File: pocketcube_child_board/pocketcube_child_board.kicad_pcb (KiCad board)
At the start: 4 copper layers, 47 x 47 mm, 17 parts, among them J1 M55-7102642R, J2 M55-7101242R, J3 M55-7101242R, J4 M55-7101242R, U1 SI3477DV-T1-GE3

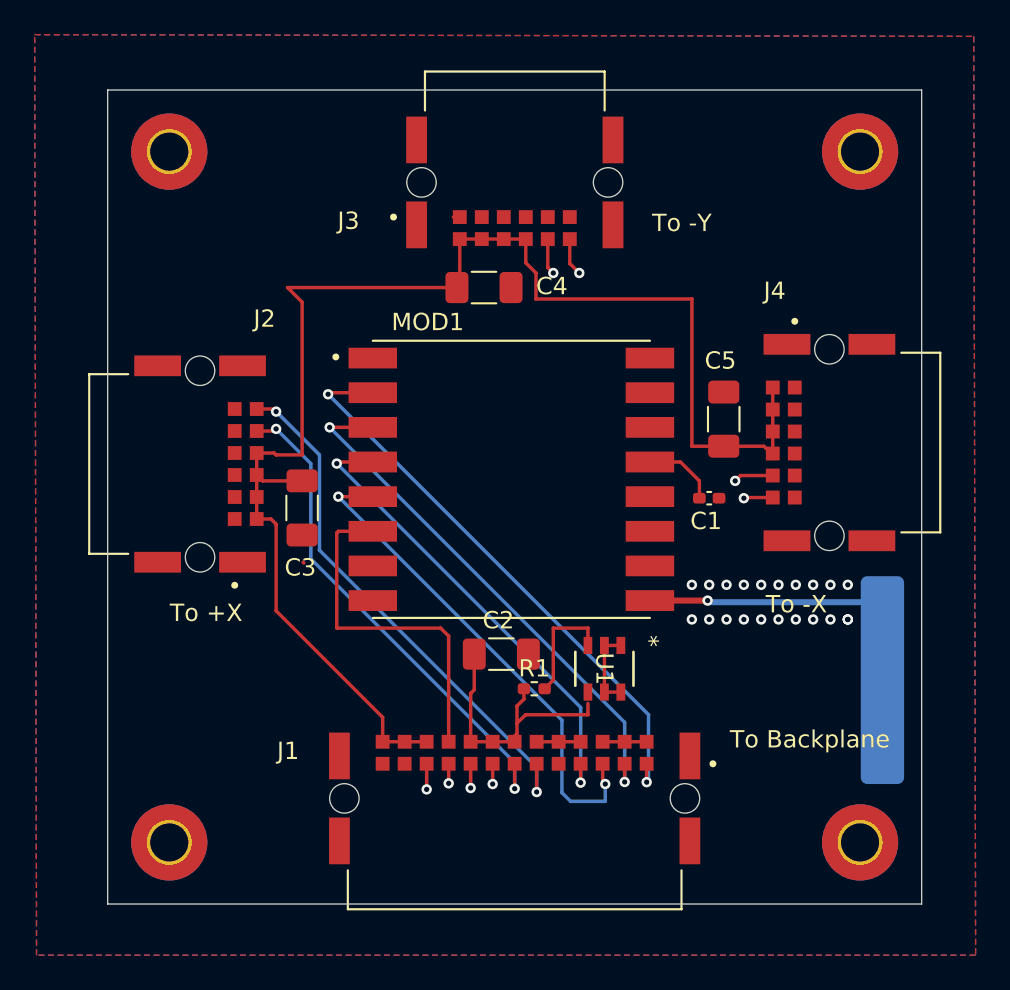
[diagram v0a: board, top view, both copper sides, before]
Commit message: Pushing Routing Changes
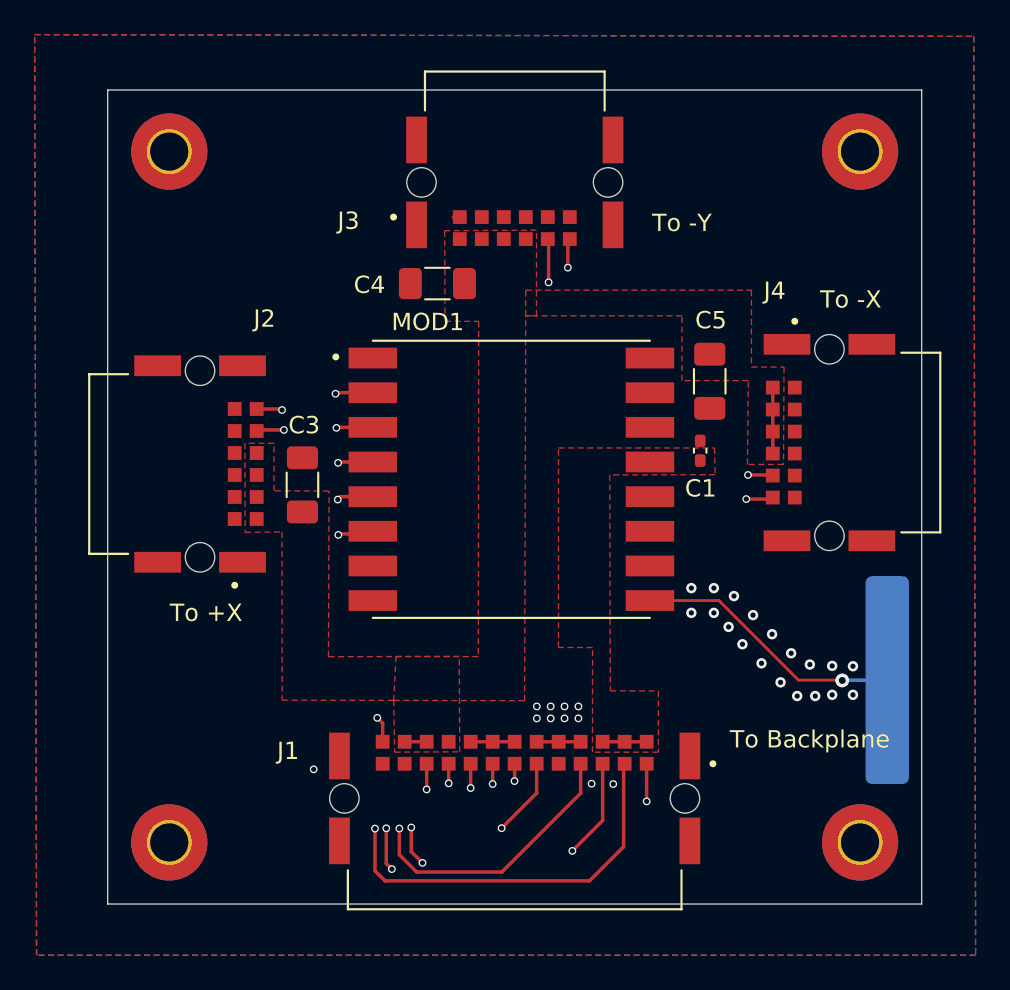
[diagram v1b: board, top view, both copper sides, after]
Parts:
- removed C2: 47uF, Capacitor_SMD:C_1206_3216Metric_Pad1.33x1.80mm_HandSolder
- removed R1: 100K, Resistor_SMD:R_0402_1005Metric_Pad0.72x0.64mm_HandSolder
- removed U1: SI3477DV-T1-GE3, inspirefly:SOT_V-T1-GE3_VIS
- moved C1 2.79 mm to (235.0, 54.8), turned to -90 degrees
- moved C4 2.70 mm to (219.8, 45.1), turned to 0 degrees
- moved C5 2.33 mm to (235.5, 50.8), turned to 90 degrees
- moved C3 1.33 mm to (212.0, 56.7), turned to -90 degrees
- moved AE1 0.28 mm to (252.5, 68.0)
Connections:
- C1 pad 2: 3.3V -> +3.3V
- J1 pad A1: ANT_SPI2_MISO -> ANT_SPI2_MOSI
- J1 pad A2: ANT_SPI2_MOSI -> ANT_SPI2_MISO
- J1 pad B10: RFM_RESET -> EXTERNAL_VOLTAGE
- J1 pad B13: EXTERNAL_VOLTAGE -> RFM_RESET
- MOD1 pad 13: 3.3V -> +3.3V
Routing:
- net EXTERNAL_VOLTAGE: track 84.5 -> 5.08 mm
- net I2C2_SDA: track 3.36 -> 45.3 mm
- net I2C2_SCL: track 3.49 -> 41.6 mm
- net I2C3_SCL: track 3.78 -> 36.6 mm
- net I2C3_SDA: track 2.82 -> 33.5 mm
- net ANT_SPI2_MOSI: track 31.1 -> 50.5 mm, vias 2 -> 4
- net ANT_SPI2_MISO: track 33.9 -> 52.6 mm
- net ANT_SPI2_SCK: track 27.5 -> 41.7 mm
- net BAT_VOLTAGE: track 15.9 -> 2.54 mm
- net I2C1_SDA: track 31.0 -> 43.2 mm
- net ANT_SPI2_NSS: track 29.4 -> 40.5 mm, vias 2 -> 4
- net I2C1_SCL: track 29.1 -> 39.6 mm
- net Net-(U1-G): track 5.71 -> 0.00 mm
- net RFM_RESET: track 20.4 -> 15.2 mm, vias 0 -> 2
- net Net-(R_BURN1-Pad1): track 4.59 -> 0.00 mm
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- added copper zone on F.Cu, net +3.3V
- added copper zone on F.Cu, net EXTERNAL_VOLTAGE
